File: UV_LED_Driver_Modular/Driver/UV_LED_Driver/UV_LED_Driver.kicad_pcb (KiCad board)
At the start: 2 copper layers, 68.6 x 30.5 mm, 11 parts, among them J1 Conn_02x06_Odd_Even, Q1 IPP80N03S4L-03

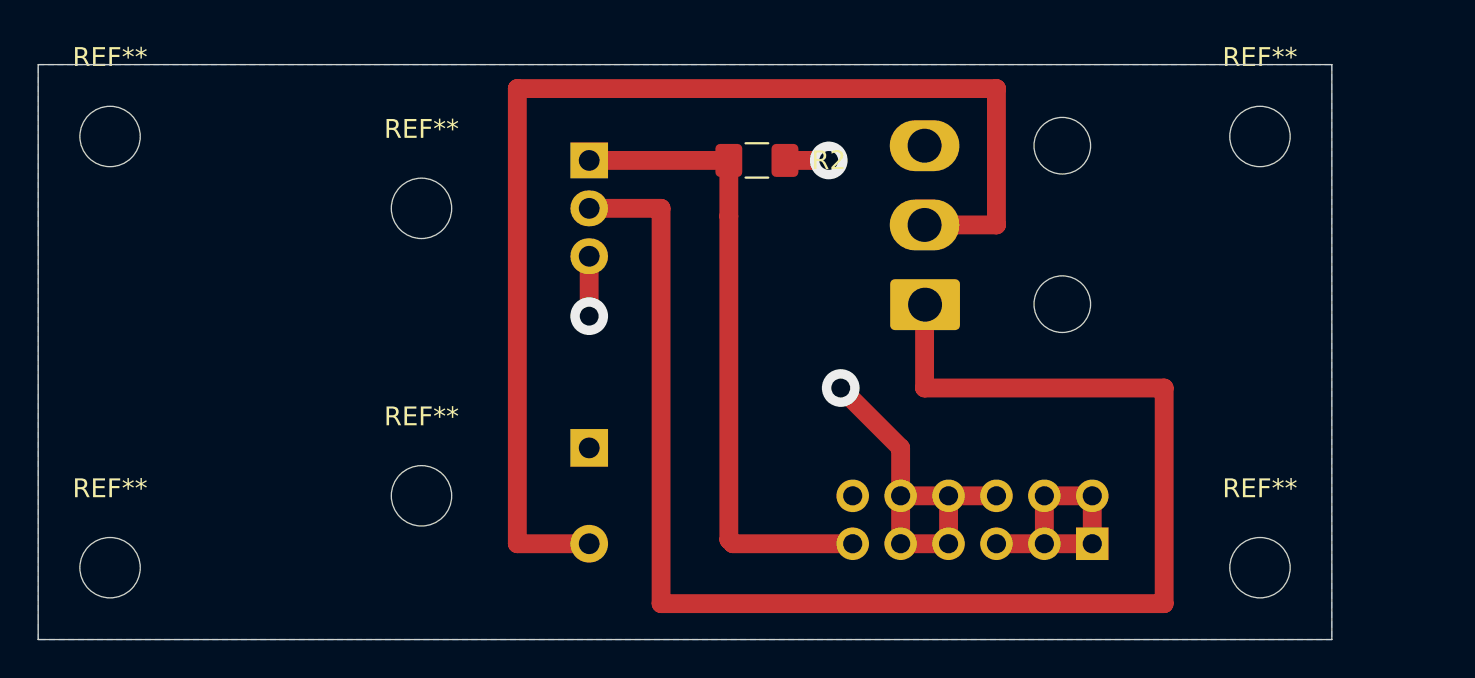
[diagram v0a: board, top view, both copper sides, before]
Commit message: docs update
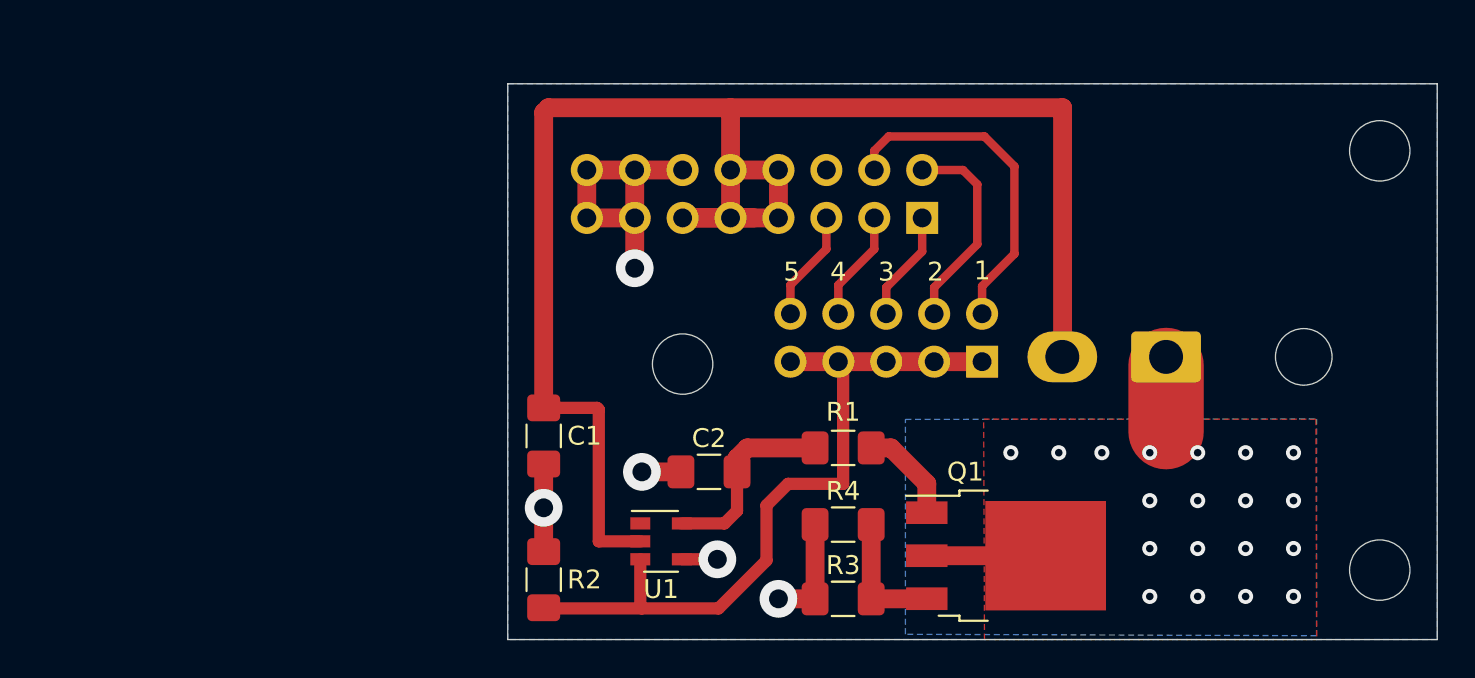
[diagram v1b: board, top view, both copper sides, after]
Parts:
- removed the REF** at (125.7, 85.1)
- removed the REF** at (125.7, 62.2)
- removed the REF** at (186.7, 62.2)
- removed the REF** at (186.7, 85.1)
- removed the REF** at (142.2, 81.3)
- removed the REF** at (142.2, 66.0)
- added C1: 1uF, Capacitor_SMD:C_1206_3216Metric_Pad1.42x1.75mm_HandSolder, F.Cu at (148.7, 78.1)
- added C2: 100nF, Capacitor_SMD:C_1206_3216Metric_Pad1.42x1.75mm_HandSolder, F.Cu at (157.5, 80.0)
- added J2: Conn_02x05_Odd_Even, Connector_PinHeader_2.54mm:PinHeader_2x05_P2.54mm_Vertical, B.Cu at (172.0, 74.2)
- added R1: 1K, Resistor_SMD:R_1206_3216Metric_Pad1.42x1.75mm_HandSolder, F.Cu at (164.6, 78.7)
- added R4: 1R, Resistor_SMD:R_1206_3216Metric_Pad1.42x1.75mm_HandSolder, F.Cu at (164.6, 82.8)
- added REF**: MountingHole_3.2mm_M3, MountingHole:MountingHole_3.2mm_M3, F.Cu at (193.0, 63.0)
- added REF**: MountingHole_3.2mm_M3, MountingHole:MountingHole_3.2mm_M3, F.Cu at (193.0, 85.2)
- added REF**: MountingHole_3.2mm_M3, MountingHole:MountingHole_3.2mm_M3, F.Cu at (156.1, 74.3)
- added U1: MCP1416, Package_TO_SOT_SMD:SOT-23-5, F.Cu at (154.9, 83.7)
- D1: footprint Connector_Molex_MiniFitJnrExtra:Molex_Mini-Fit_Jr_5569-06A2_2x03_P4.20mm_Horizontal -> Connector_Molex:Molex_Mini-Fit_Jr_5569-02A2_2x01_P4.20mm_Horizontal
- J1: value Conn_02x06_Odd_Even -> Conn_02x08_Odd_Even; footprint Connector_IDC:IDC-Header_2x06_P2.54mm_Vertical -> Connector_PinHeader_2.54mm:PinHeader_2x08_P2.54mm_Vertical
- Q1: value IPP80N03S4L-03 -> NTD60N02R; footprint Package_TO_SOT_THT:TO-220-3_Vertical -> Package_TO_SOT_SMD:TO-252-3_TabPin2; moved to F.Cu
- R3: value R100 -> 1R; footprint Package_TO_SOT_THT:TO-220-2_Vertical -> Resistor_SMD:R_1206_3216Metric_Pad1.42x1.75mm_HandSolder; moved to F.Cu
- moved Q1 30.5 mm to (173.2, 84.5), turned to 0 degrees
- moved R2 24.9 mm to (148.7, 85.7), turned to 270 degrees
- moved J1 19.5 mm to (168.8, 66.5)
- moved R3 15.7 mm to (164.6, 86.7), turned to 180 degrees
- moved D1 13.1 mm to (181.7, 73.9)
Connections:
- D1 pad 2: /UV_LED_DRIVER_MODULE/LED_ANODE_OUT -> VPP
- J1 pad 1: +5V -> /LED_PWM_OUT3
- J1 pad 10: GNDS -> VPP
- J1 pad 11: /UV_PWM -> VPP
- J1 pad 12: Net-(J1-Pad12) -> GNDS
- J1 pad 2: +5V -> /LED_PWM_OUT2
- J1 pad 3: +5V -> /LED_PWM_OUT4
- J1 pad 4: +5V -> /LED_PWM_OUT1
- J1 pad 5: +5V -> /LED_PWM_OUT5
- J1 pad 6: GNDS -> Net-(J1-Pad6)
- J1 pad 7: GNDS -> VPP
- J1 pad 8: GNDS -> VPP
- J1 pad 9: GNDS -> VPP
- Q1 pad 1: /UV_PWM -> Net-(Q1-Pad1)
- Q1 pad 3: GNDS -> Net-(Q1-Pad3)
- R3 pad 1: /UV_LED_DRIVER_MODULE/+5V -> Net-(Q1-Pad3)
- R3 pad 2: /UV_LED_DRIVER_MODULE/LED_ANODE_OUT -> GNDS
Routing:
- net VPP: track 0.00 -> 89.0 mm
- net /UV_LED_DRIVER_MODULE/LED_CATHODE_OUT: track 80.0 -> 11.7 mm, vias 0 -> 19
- net /UV_LED_DRIVER_MODULE/LED_ANODE_OUT: track 64.4 -> 0.00 mm
- net /LED_PWM_OUT1: track 0.00 -> 17.9 mm
- net +5V: track 12.7 -> 0.00 mm
- net /LED_PWM_OUT2: track 0.00 -> 11.0 mm
- net Net-(C2-Pad1): track 0.00 -> 10.4 mm
- net Net-(Q1-Pad3): track 0.00 -> 6.89 mm
- net /UV_PWM: track 34.2 -> 40.1 mm
- net /LED_PWM_OUT5: track 0.00 -> 5.87 mm
- net /LED_PWM_OUT4: track 0.00 -> 5.87 mm
- net /LED_PWM_OUT3: track 0.00 -> 5.87 mm
- net Net-(Q1-Pad1): track 0.00 -> 5.27 mm
- net GNDS: track 25.2 -> 29.8 mm, vias 3 -> 5
- added copper zone on B.Cu, net /UV_LED_DRIVER_MODULE/LED_CATHODE_OUT
- added copper zone on F.Cu, net /UV_LED_DRIVER_MODULE/LED_CATHODE_OUT
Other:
- board size 68.6 x 30.5 mm -> 49.3 x 29.5 mm
- board text added: "1"
- board text added: "2"
- board text added: "3"
- board text added: "4"
- board text added: "5"
